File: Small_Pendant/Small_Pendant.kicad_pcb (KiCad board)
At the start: 4 copper layers, 28 x 28 mm, 205 parts, among them J1 USB_C_Receptacle_USB2.0_16P, U1 FT234XD-R, U2 SN74LVC1T45DCK

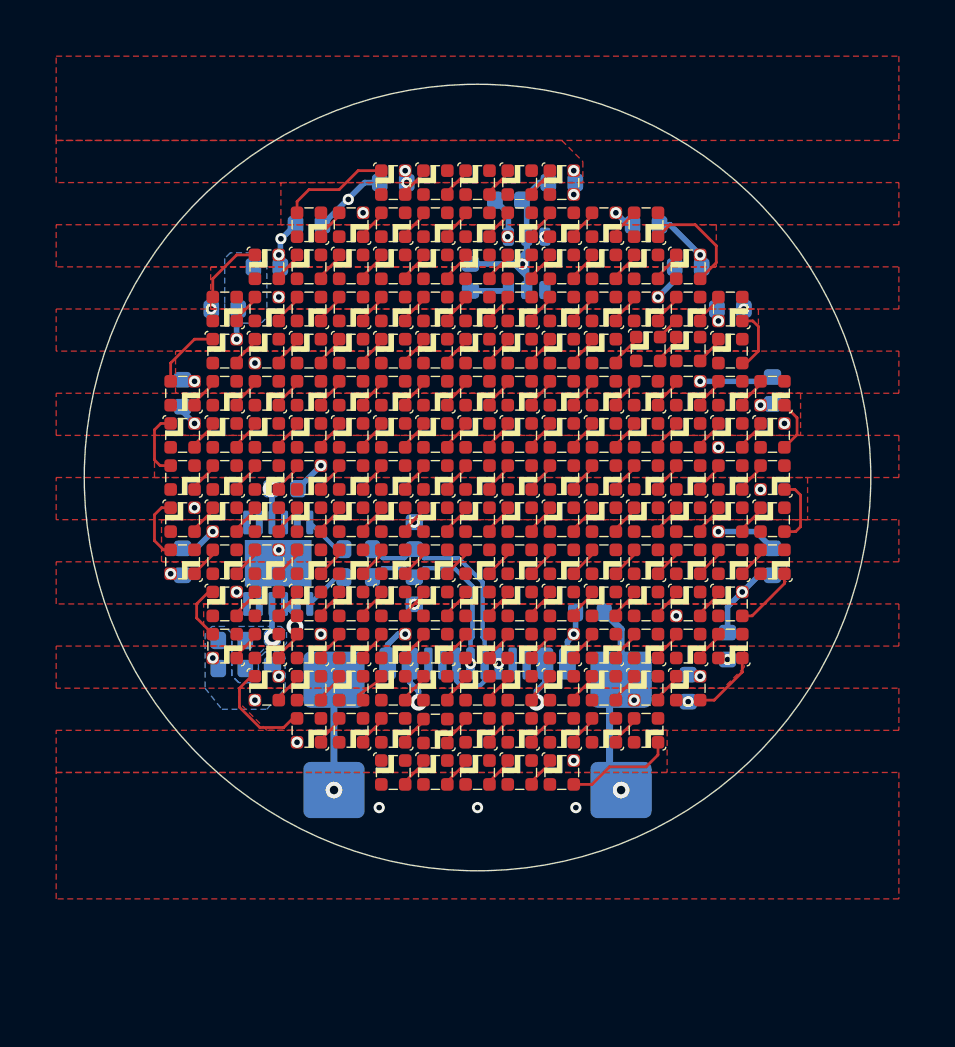
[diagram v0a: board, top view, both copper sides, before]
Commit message: [HW] Make 'lollipop' shaped for USB connector
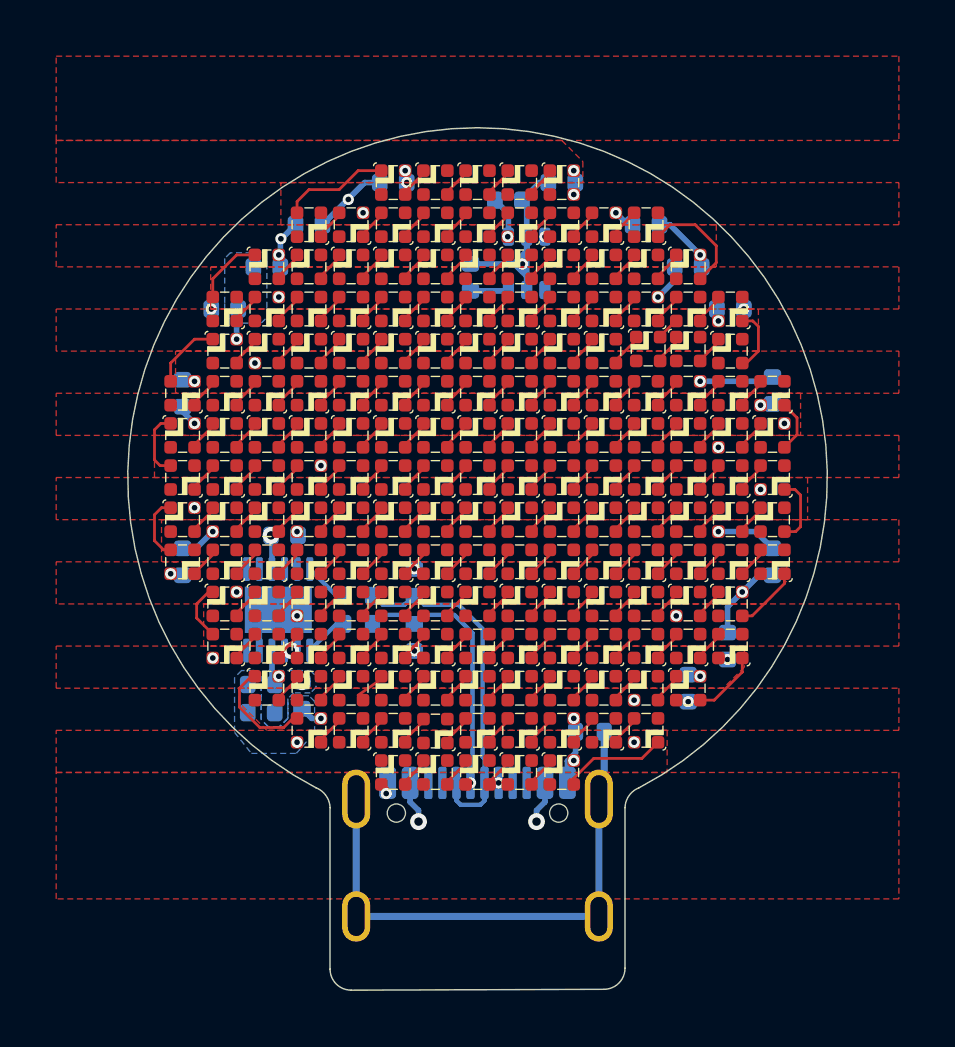
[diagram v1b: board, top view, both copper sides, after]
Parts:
- J1: footprint Connector_USB:USB_C_Receptacle_GCT_USB4110 -> Connector_USB:USB_C_Receptacle_GCT_USB4105-xx-A_16P_TopMnt_Horizontal
- moved J1 4.25 mm to (50.0, 64.5)
- moved R1 4.25 mm to (54.0, 59.0)
- moved C24 1.89 mm to (42.3, 57.4)
- moved C25 1.89 mm to (42.3, 58.4)
- moved C26 1.89 mm to (43.8, 57.8)
- moved C23 1.66 mm to (43.1, 52.1)
- moved R2 1.66 mm to (45.8, 55.2)
- moved R3 1.66 mm to (45.8, 54.2)
- moved U1 1.66 mm to (42.9, 54.7)
- moved C21 1.66 mm to (47.8, 55.7)
- moved C22 1.66 mm to (47.8, 53.7)
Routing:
- net +3V3_USB: track 9.19 -> 6.01 mm
- net USB_D+: track 9.87 -> 12.5 mm
- net USB_D-: track 9.28 -> 11.9 mm
- net VUSB: track 14.8 -> 16.2 mm
- net Earth: track 23.8 -> 23.1 mm, vias 30 -> 27
- net Net-(J1-SHIELD): track 19.9 -> 19.5 mm, vias 2 -> 0
- net +5V: vias 21 -> 22
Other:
- board size 28 x 28 mm -> 24.9 x 30.7 mm
